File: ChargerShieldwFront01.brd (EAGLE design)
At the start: 158.8 x 147.3 mm, 91 parts, among them IC1 TL431, IC2 LM324N, Q1 BUZ11BH, Q2 BD648, Q3 BUZ171, Q4 BUZ11BH, Q5 BD648, Q6 BUZ171, T1 BC548, T2 BC548, X1 +5V, X2 VCC, X3 Battery, X4 Battery

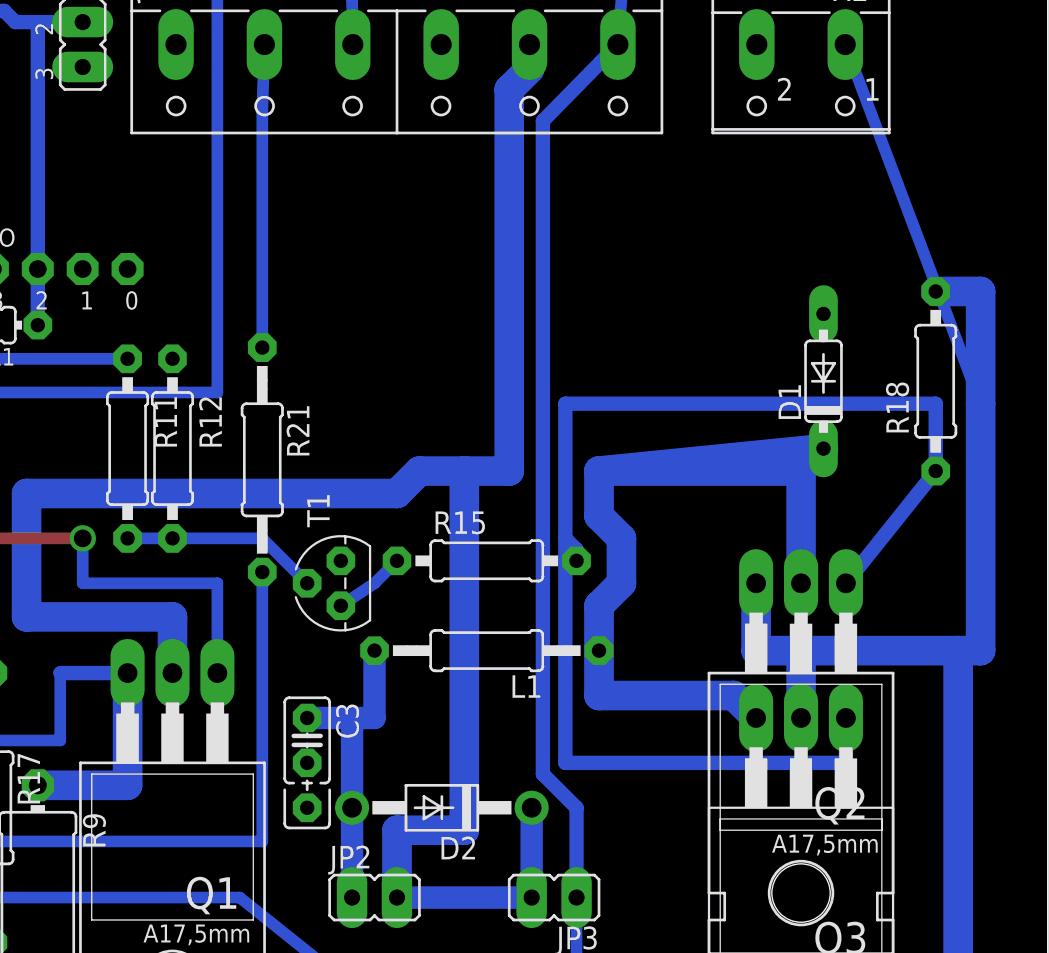
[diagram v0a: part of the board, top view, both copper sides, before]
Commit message: arrangement
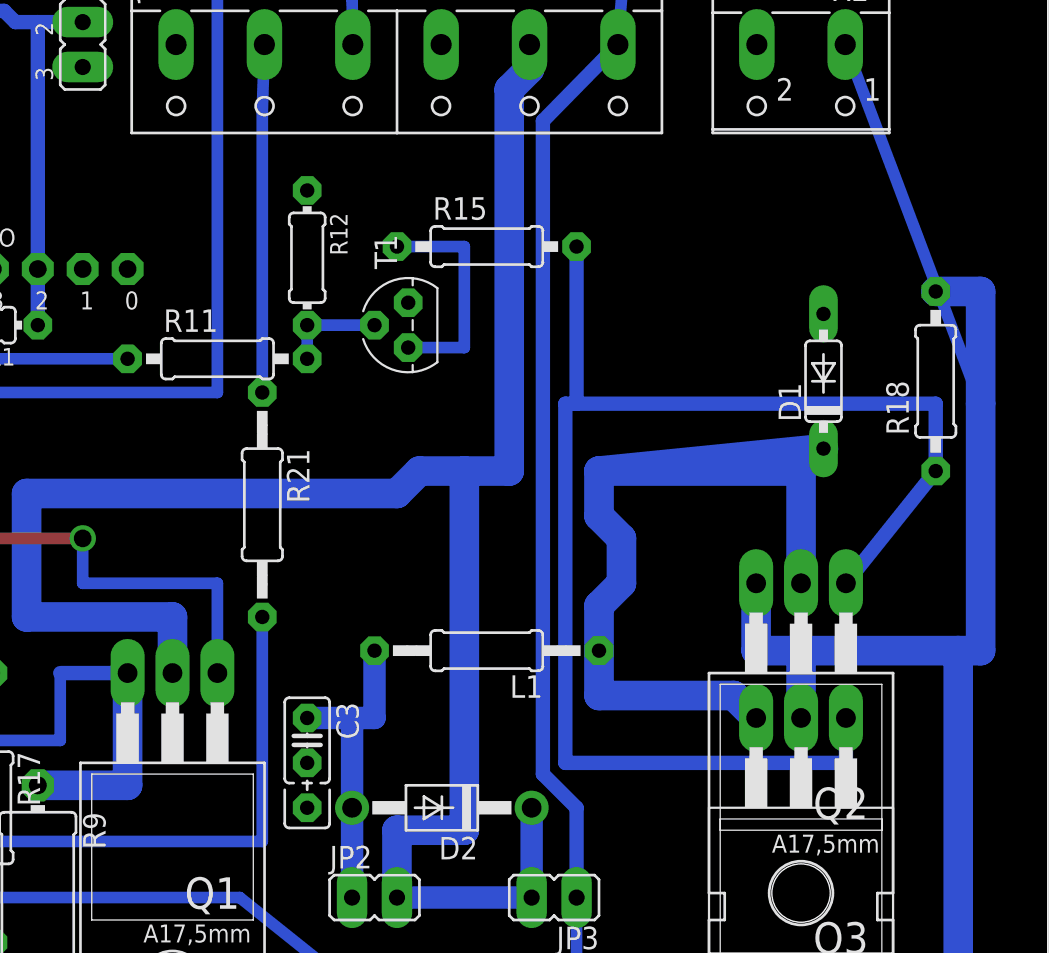
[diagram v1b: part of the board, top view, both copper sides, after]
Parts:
- R12: device rcl:0207/10 -> rcl:0204/7
- moved R15 17.8 mm to (83.8, 52.1)
- moved T1 15.1 mm to (79.4, 47.6)
- moved R12 13.2 mm to (73.7, 51.4)
- moved R11 7.18 mm to (68.6, 45.7), turned to 0 degrees
- moved R21 2.54 mm to (71.1, 37.5)
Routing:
- net N$6: track 4.09 -> 12.7 mm
- net N$7: track 73.2 -> 80.5 mm
- net N$5: track 11.2 -> 5.72 mm
- net N$14: track 61.4 -> 58.8 mm
- net I1_SENSE-: track 17.3 -> 19.8 mm
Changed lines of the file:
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@@
 <setting verticaltext="up"/>
 </settings>
-<grid distance="0.05" unitdist="inch" unit="mm" style="lines" multiple="1" display="yes" altdistance="0.025" altunitdist="inch" altunit="mm"/>
+<grid distance="2.54" unitdist="mm" unit="mm" style="lines" multiple="1" display="yes" altdistance="1.27" altunitdist="mm" altunit="mm"/>
 <layers>
 <layer number="1" name="Top" color="4" fill="1" visible="yes" active="yes"/>
@@
 <element name="S1" library="SparkFun-Electromechanical" package="TACTILE-PTH" value="Down" x="46.99" y="97.79" rot="R90"/>
 <element name="S2" library="SparkFun-Electromechanical" package="TACTILE-PTH" value="Up" x="39.37" y="97.79" rot="R90"/>
-<element name="T1" library="transistor" package="TO92" value="BC548" x="75.565" y="33.02" rot="R90"/>
-<element name="R11" library="rcl" package="0207/10" value="2k2" x="63.5" y="40.64" rot="R270"/>
-<element name="R15" library="rcl" package="0207/10" value="1k" x="83.82" y="34.29"/>
+<element name="T1" library="transistor" package="TO92" value="BC548" x="79.375" y="47.625" rot="R90"/>
+<element name="R11" library="rcl" package="0207/10" value="2k2" x="68.58" y="45.72"/>
+<element name="R15" library="rcl" package="0207/10" value="1k" x="83.82" y="52.07"/>
 <element name="C3" library="rcl" package="C025_050-025X075" value="15n/60V" x="73.66" y="24.13" rot="R270"/>
 <element name="R18" library="rcl" package="0207/10" value="1k" x="109.22" y="44.45" rot="R90"/>
@@
 <element name="IC2" library="linear" package="DIL14" value="LM324N" x="26.67" y="24.13" rot="R90"/>
 <element name="R20" library="rcl" package="0204/7" value="100k" x="33.655" y="12.7" rot="R270"/>
-<element name="R21" library="rcl" package="0207/12" value="10k" x="71.12" y="40.005" rot="R270"/>
+<element name="R21" library="rcl" package="0207/12" value="10k" x="71.12" y="37.465" rot="R270"/>
 <element name="R9" library="rcl" package="0414/15" value="1R666" x="58.42" y="13.97" rot="R270"/>
-<element name="R12" library="rcl" package="0207/10" value="100k" x="66.04" y="40.64" rot="R270"/>
+<element name="R12" library="rcl" package="0204/7" value="100k" x="73.66" y="51.435" rot="R270"/>
 <element name="R19" library="rcl" package="0207/12" value="1k" x="46.99" y="12.065" rot="R180"/>
 <element name="R24" library="rcl" package="0207/10" value="100k" x="50.8" y="19.05" rot="R270"/>
@@
 <contactref element="T1" pad="2"/>
 <contactref element="R12" pad="2"/>
-<wire x1="63.5" y1="35.56" x2="66.04" y2="35.56" width="0.6604" layer="16"/>
-<wire x1="66.04" y1="35.56" x2="71.12" y2="35.56" width="0.6604" layer="16"/>
-<wire x1="71.12" y1="35.56" x2="73.66" y2="33.02" width="0.6604" layer="16"/>
+<wire x1="73.66" y1="45.72" x2="73.66" y2="47.625" width="0.6604" layer="16"/>
+<wire x1="73.66" y1="47.625" x2="77.47" y2="47.625" width="0.6604" layer="16"/>
 </signal>
 <signal name="N$6">
 <contactref element="T1" pad="3"/>
 <contactref element="R15" pad="1"/>
-<wire x1="78.74" y1="34.29" x2="77.47" y2="33.02" width="0.6604" layer="16"/>
-<wire x1="77.47" y1="33.02" x2="75.565" y2="31.75" width="0.6604" layer="16"/>
+<wire x1="78.74" y1="52.07" x2="82.55" y2="52.07" width="0.6604" layer="16"/>
+<wire x1="82.55" y1="52.07" x2="82.55" y2="46.355" width="0.6604" layer="16"/>
+<wire x1="82.55" y1="46.355" x2="79.375" y2="46.355" width="0.6604" layer="16"/>
 </signal>
 <signal name="N$7">
@@
 <wire x1="104.14" y1="22.86" x2="104.14" y2="25.4" width="0.8128" layer="16"/>
 <wire x1="88.265" y1="22.86" x2="104.14" y2="22.86" width="0.8128" layer="16"/>
-<wire x1="88.265" y1="43.18" x2="88.265" y2="35.56" width="0.8128" layer="16"/>
-<wire x1="88.265" y1="35.56" x2="88.265" y2="22.86" width="0.8128" layer="16"/>
-<wire x1="109.22" y1="43.18" x2="88.265" y2="43.18" width="0.8128" layer="16"/>
+<wire x1="88.265" y1="43.18" x2="88.265" y2="22.86" width="0.8128" layer="16"/>
+<wire x1="109.22" y1="43.18" x2="88.9" y2="43.18" width="0.8128" layer="16"/>
+<wire x1="88.9" y1="43.18" x2="88.265" y2="43.18" width="0.8128" layer="16"/>
 <wire x1="109.22" y1="43.18" x2="109.22" y2="39.37" width="0.8128" layer="16"/>
 <wire x1="109.22" y1="39.37" x2="104.14" y2="33.02" width="0.8128" layer="16"/>
-<wire x1="88.9" y1="34.29" x2="88.9" y2="34.925" width="0.8128" layer="16"/>
-<wire x1="88.9" y1="34.925" x2="88.265" y2="35.56" width="0.8128" layer="16"/>
+<wire x1="88.9" y1="52.07" x2="88.9" y2="43.18" width="0.8128" layer="16"/>
 </signal>
 <signal name="VCC">
@@
 <wire x1="31.75" y1="19.05" x2="30.48" y2="19.05" width="0.6604" layer="16"/>
 <wire x1="33.02" y1="17.78" x2="33.655" y2="16.51" width="0.6604" layer="16"/>
-<wire x1="71.12" y1="18.415" x2="71.12" y2="33.655" width="0.6604" layer="16"/>
+<wire x1="71.12" y1="18.415" x2="71.12" y2="31.115" width="0.6604" layer="16"/>
 <wire x1="47.625" y1="18.415" x2="71.12" y2="18.415" width="0.6604" layer="16"/>
 <wire x1="43.18" y1="13.97" x2="47.625" y2="18.415" width="0.6604" layer="16"/>
@@
 <contactref element="R21" pad="1"/>
 <contactref element="X3" pad="5"/>
-<wire x1="71.12" y1="59.69" x2="71.12" y2="46.355" width="0.6604" layer="16"/>
+<wire x1="71.12" y1="59.69" x2="71.12" y2="43.815" width="0.6604" layer="16"/>
 <wire x1="71.24" y1="63.5" x2="71.12" y2="59.69" width="0.6604" layer="16"/>
 <wire x1="71.12" y1="63.5" x2="71.24" y2="63.5" width="0.6604" layer="16"/>
